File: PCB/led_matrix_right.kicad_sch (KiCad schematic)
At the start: 39 parts

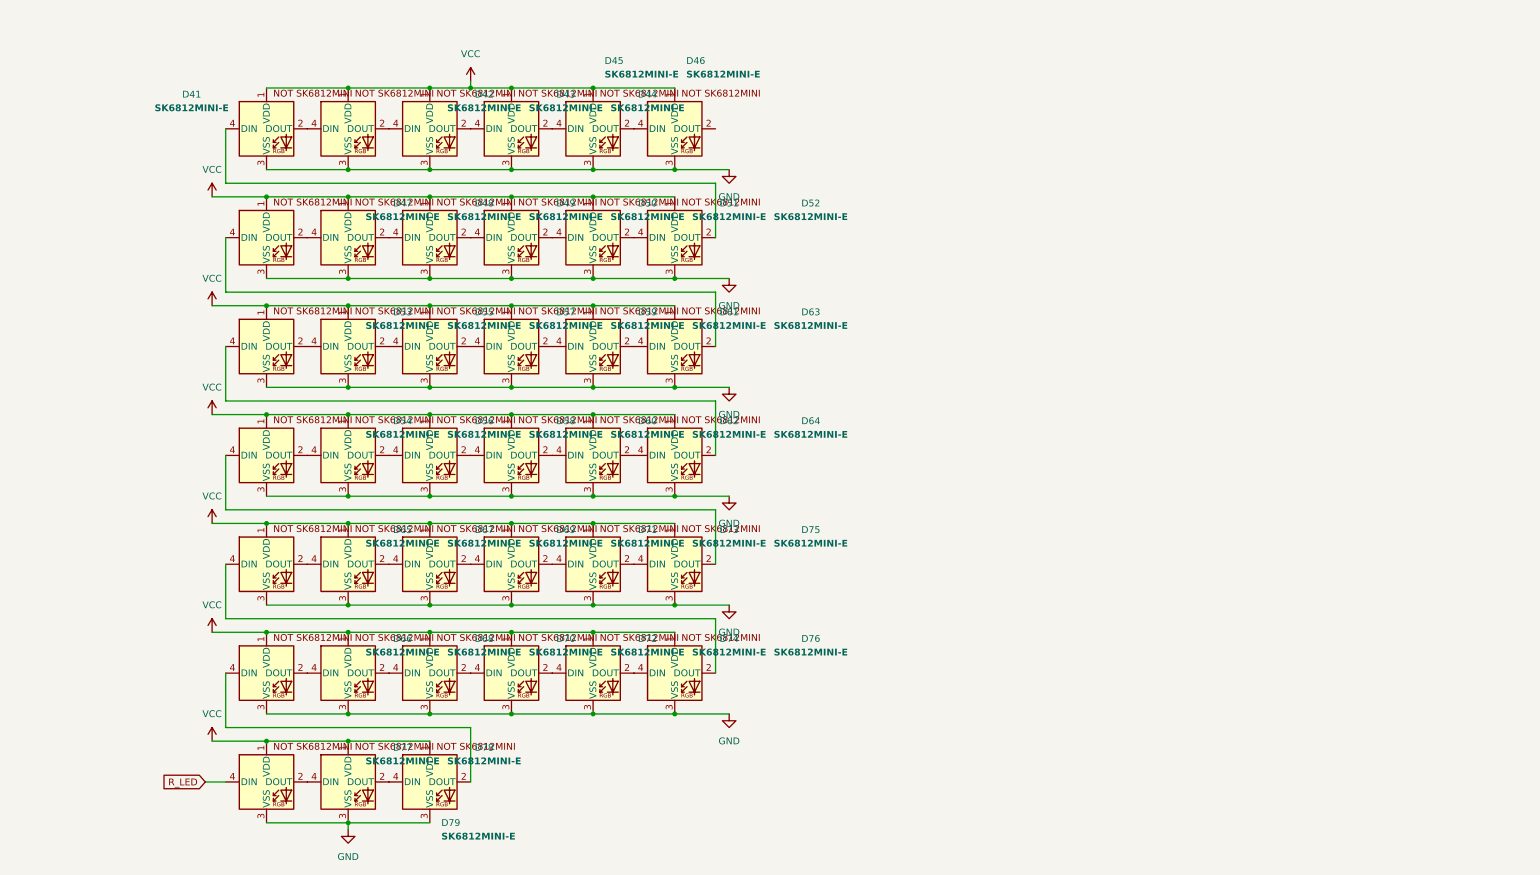
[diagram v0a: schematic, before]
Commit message: redid the leds
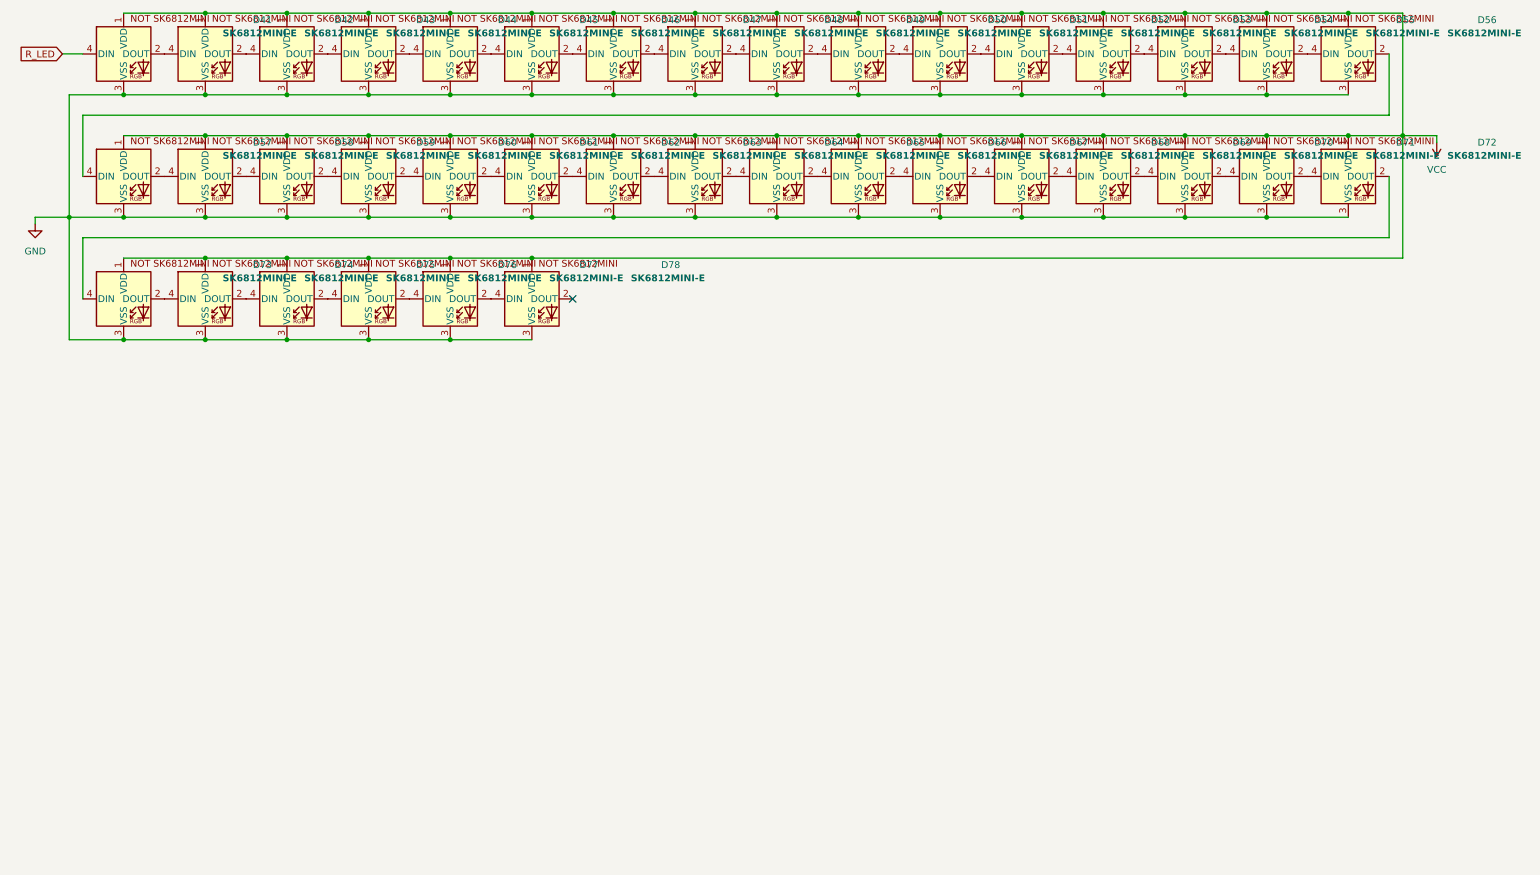
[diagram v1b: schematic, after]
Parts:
- removed D79: SK6812MINI-E, footprints:SK6812MINI-E_fixed, symbol SK6812MINI-E:SK6812MINI-E
- D41, D42, D43, D44, D45, D46, D47, D48, D49, D50, D51, D52, D53, D54, D55, D56, D57, D58, D59, D60, D61, D62, D63, D64, D65, D66, D67, D68, D69, D70, D71, D72, D73, D74, D75, D76, D77, D78: footprint footprints:SK6812MINI-E_fixed -> SK6812MINI-E - 3.2x2.8x1.78mm
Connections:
- net R_LED: now also D41.4 (DIN); no longer D77.4 (DIN)
- net at D66.2 (DOUT): now also D67.4 (DIN); no longer D68.4 (DIN)
- net at D66.4 (DIN): now also D65.2 (DOUT)
- net at D76.2 (DOUT): now also D77.4 (DIN); no longer D65.4 (DIN)
- net at D74.2 (DOUT): now also D75.4 (DIN); no longer D76.4 (DIN)
- net at D71.2 (DOUT): now also D72.4 (DIN); no longer D73.4 (DIN)
- net at D71.4 (DIN): now also D70.2 (DOUT); no longer D69.2 (DOUT)
- net at D64.4 (DIN): now also D63.2 (DOUT); no longer D62.2 (DOUT)
- net at D62.4 (DIN): now also D61.2 (DOUT); no longer D60.2 (DOUT)
- net at D47.4 (DIN): now also D46.2 (DOUT); no longer D63.2 (DOUT)
- net at D53.4 (DIN): now also D52.2 (DOUT); no longer D64.2 (DOUT)
- net at D70.4 (DIN): now also D69.2 (DOUT); no longer D68.2 (DOUT)
- net at D73.2 (DOUT): now also D74.4 (DIN); no longer D75.4 (DIN)
- net at D67.2 (DOUT): now also D68.4 (DIN); no longer D69.4 (DIN)
- net at D63.4 (DIN): now also D62.2 (DOUT); no longer D61.2 (DOUT)
- net at D58.2 (DOUT): now also D59.4 (DIN); no longer D60.4 (DIN)
- net at D56.2 (DOUT): now also D57.4 (DIN); no longer D58.4 (DIN)
- net at D55.2 (DOUT): now also D56.4 (DIN); no longer D57.4 (DIN)
- net at D55.4 (DIN): now also D54.2 (DOUT); no longer D53.2 (DOUT)
- net at D61.4 (DIN): now also D60.2 (DOUT); no longer D59.2 (DOUT)
- net at D57.2 (DOUT): now also D58.4 (DIN); no longer D59.4 (DIN)
- net at D72.2 (DOUT): now also D73.4 (DIN); no longer D74.4 (DIN)
- net at D75.2 (DOUT): now also D76.4 (DIN); no longer D54.4 (DIN)
- new net: D53.2 (DOUT), D54.4 (DIN)
- new net: D64.2 (DOUT), D65.4 (DIN)
- new net: D59.2 (DOUT), D60.4 (DIN)
- new net: D68.2 (DOUT), D69.4 (DIN)
- no-connect marks 0 -> 1
